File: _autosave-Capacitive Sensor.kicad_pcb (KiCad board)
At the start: 2 copper layers, 25 x 60.2 mm, 7 parts, among them J1 Conn_01x03, U1 TLC555

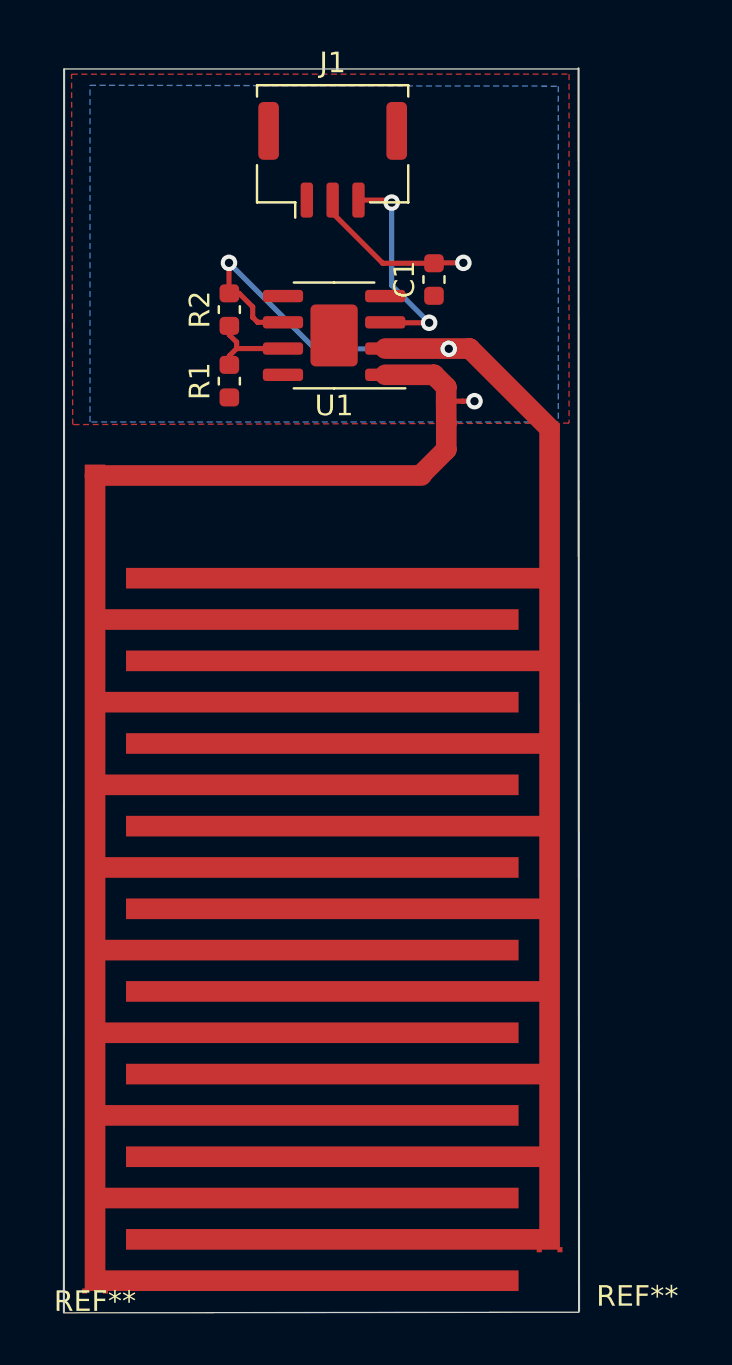
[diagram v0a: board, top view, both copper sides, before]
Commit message: update sensor
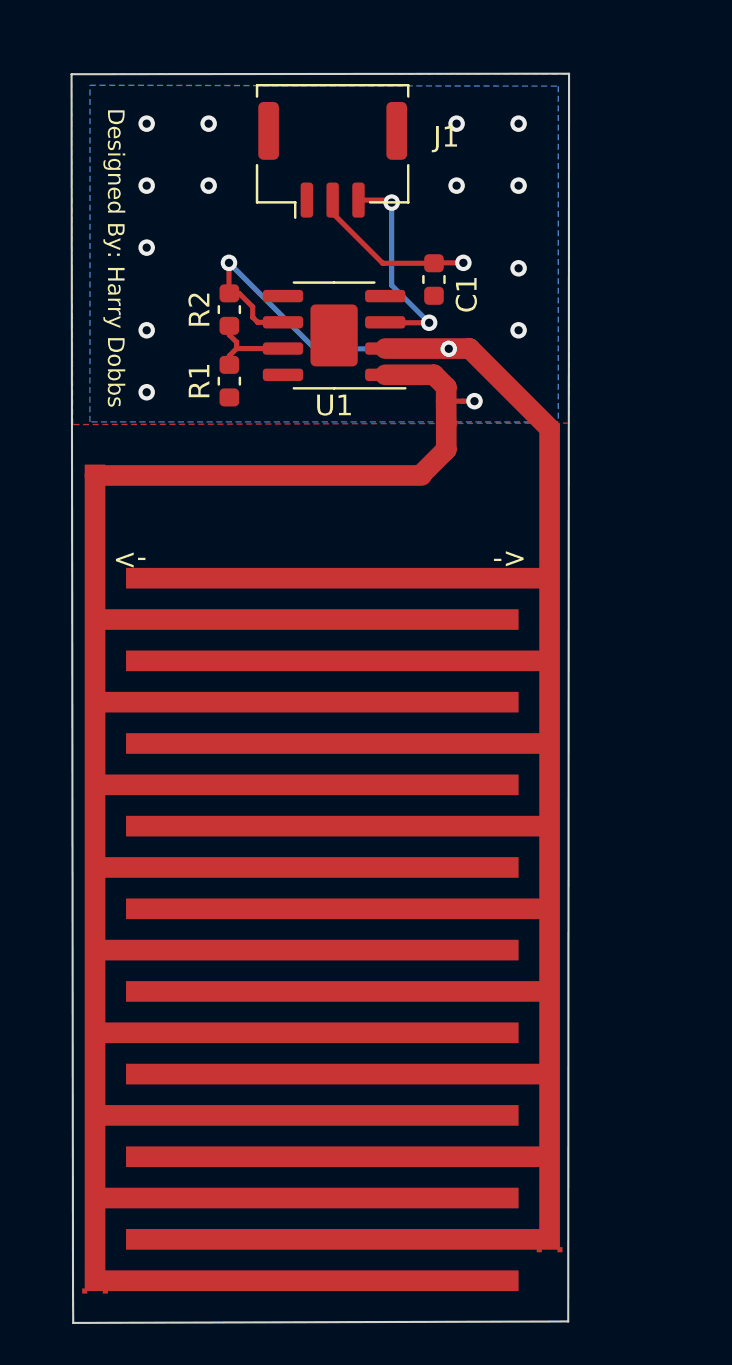
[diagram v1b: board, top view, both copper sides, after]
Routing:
- net C-: vias 2 -> 15
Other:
- board size 25 x 60.2 mm -> 24.1 x 60.5 mm
- board text added: "->"
- board text added: "Designed By: Harry Dobbs"
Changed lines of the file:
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@@
   (general
     (thickness 1.6)
-    (drawings 4)
-    (tracks 49)
+    (drawings 9)
+    (tracks 62)
     (zones 0)
     (modules 7)
@@
   )
   (setup
-    (last_trace_width 0.25)
+    (last_trace_width 1)
     (user_trace_width 0.25)
     (user_trace_width 1)
@@
     (solder_mask_min_width 0.25)
     (aux_axis_origin 0 0)
-    (visible_elements FFFBEF7F)
+    (visible_elements FFFFEF7F)
     (pcbplotparams
       (layerselection 0x010fc_ffffffff)
@@
   (module muwave_polygon (layer F.Cu)
     (at 160.5 141.5 180)
-    (fp_text reference REF** (at -4.25 -2.25) (layer F.SilkS)
-      (effects (font (size 1 1) (thickness 0.15)))
-    )
-    (fp_text value muwave_polygon (at -2.75 -3.5) (layer F.Fab)
+    (fp_text reference REF** (at 3.5 -2) (layer F.SilkS) hide
+      (effects (font (size 1 1) (thickness 0.15)))
+    )
+    (fp_text value muwave_polygon (at -10.78744 -4.41792) (layer F.Fab)
       (effects (font (size 1 1) (thickness 0.15)))
     )
@@
   (module muwave_polygon (layer F.Cu)
     (at 138.5 143.5)
-    (fp_text reference REF** (at 0 0.5) (layer F.SilkS)
-      (effects (font (size 1 1) (thickness 0.15)))
-    )
-    (fp_text value muwave_polygon (at 0 -0.5) (layer F.Fab)
+    (fp_text reference REF** (at 0 0.5) (layer F.SilkS) hide
+      (effects (font (size 1 1) (thickness 0.15)))
+    )
+    (fp_text value muwave_polygon (at -13 -1.5) (layer F.Fab)
       (effects (font (size 1 1) (thickness 0.15)))
     )
@@
     (tags "connector Molex CLIK-Mate side entry")
     (attr smd)
-    (fp_text reference J1 (at 0 -4.7) (layer F.SilkS)
+    (fp_text reference J1 (at 5.50896 -1.09968) (layer F.SilkS)
       (effects (font (size 1 1) (thickness 0.15)))
     )
@@
     (tags capacitor)
     (attr smd)
-    (fp_text reference C1 (at 0 -1.43 90) (layer F.SilkS)
+    (fp_text reference C1 (at -0.71638 1.6002 90) (layer F.SilkS)
       (effects (font (size 1 1) (thickness 0.15)))
     )
@@
       (effects (font (size 1 1) (thickness 0.15)))
     )
+    (fp_line (start -0.8 0.4) (end -0.8 -0.4) (layer F.Fab) (width 0.1))
+    (fp_line (start -0.8 -0.4) (end 0.8 -0.4) (layer F.Fab) (width 0.1))
+    (fp_line (start 0.8 -0.4) (end 0.8 0.4) (layer F.Fab) (width 0.1))
+    (fp_line (start 0.8 0.4) (end -0.8 0.4) (layer F.Fab) (width 0.1))
+    (fp_line (start -0.162779 -0.51) (end 0.162779 -0.51) (layer F.SilkS) (width 0.12))
+    (fp_line (start -0.162779 0.51) (end 0.162779 0.51) (layer F.SilkS) (width 0.12))
+    (fp_line (start -1.48 0.73) (end -1.48 -0.73) (layer F.CrtYd) (width 0.05))
+    (fp_line (start -1.48 -0.73) (end 1.48 -0.73) (layer F.CrtYd) (width 0.05))
+    (fp_line (start 1.48 -0.73) (end 1.48 0.73) (layer F.CrtYd) (width 0.05))
+    (fp_line (start 1.48 0.73) (end -1.48 0.73) (layer F.CrtYd) (width 0.05))
     (fp_text user %R (at 0.5 -1 90) (layer F.Fab)
       (effects (font (size 0.4 0.4) (thickness 0.06)))
     )
-    (fp_line (start 1.48 0.73) (end -1.48 0.73) (layer F.CrtYd) (width 0.05))
-    (fp_line (start 1.48 -0.73) (end 1.48 0.73) (layer F.CrtYd) (width 0.05))
-    (fp_line (start -1.48 -0.73) (end 1.48 -0.73) (layer F.CrtYd) (width 0.05))
-    (fp_line (start -1.48 0.73) (end -1.48 -0.73) (layer F.CrtYd) (width 0.05))
-    (fp_line (start -0.162779 0.51) (end 0.162779 0.51) (layer F.SilkS) (width 0.12))
-    (fp_line (start -0.162779 -0.51) (end 0.162779 -0.51) (layer F.SilkS) (width 0.12))
-    (fp_line (start 0.8 0.4) (end -0.8 0.4) (layer F.Fab) (width 0.1))
-    (fp_line (start 0.8 -0.4) (end 0.8 0.4) (layer F.Fab) (width 0.1))
-    (fp_line (start -0.8 -0.4) (end 0.8 -0.4) (layer F.Fab) (width 0.1))
-    (fp_line (start -0.8 0.4) (end -0.8 -0.4) (layer F.Fab) (width 0.1))
+    (pad 1 smd roundrect (at -0.7875 0 90) (size 0.875 0.95) (layers F.Cu F.Paste F.Mask) (roundrect_rratio 0.25)
+      (net 2 +3V3))
     (pad 2 smd roundrect (at 0.7875 0 90) (size 0.875 0.95) (layers F.Cu F.Paste F.Mask) (roundrect_rratio 0.25)
       (net 1 C-))
-    (pad 1 smd roundrect (at -0.7875 0 90) (size 0.875 0.95) (layers F.Cu F.Paste F.Mask) (roundrect_rratio 0.25)
-      (net 2 +3V3))
     (model ${KISYS3DMOD}/Capacitor_SMD.3dshapes/C_0603_1608Metric.wrl
       (at (xyz 0 0 0))
@@
     )
   )
-  (gr_line (start 136.99236 84.3534) (end 161.8996 84.3534) (layer Edge.Cuts) (width 0.05))
-  (gr_line (start 136.96696 144.55648) (end 161.91992 144.526) (layer Edge.Cuts) (width 0.05))
-  (gr_line (start 161.8996 84.32292) (end 161.925 144.47012) (layer Edge.Cuts) (width 0.1))
-  (gr_line (start 136.99236 144.50568) (end 137.00252 84.36864) (layer Edge.Cuts) (width 0.1))
+  (gr_text -> (at 140.18768 108.1532 180) (layer F.SilkS)
+    (effects (font (size 1 1) (thickness 0.15)))
+  )
+  (gr_text -> (at 158.56204 108.0262) (layer F.SilkS)
+    (effects (font (size 1 1) (thickness 0.15)))
+  )
+  (gr_text "Designed By: Harry Dobbs " (at 139.5 93.5 270) (layer F.SilkS)
+    (effects (font (size 0.8 0.8) (thickness 0.15)))
+  )
+  (gr_line (start 137.44448 145.04416) (end 137.43432 143.62176) (layer Edge.Cuts) (width 0.1))
+  (gr_line (start 161.40176 144.97304) (end 137.44448 145.04416) (layer Edge.Cuts) (width 0.1))
+  (gr_line (start 161.4424 84.582) (end 161.40176 144.97304) (layer Edge.Cuts) (width 0.1))
+  (gr_line (start 137.3632 84.6074) (end 161.4424 84.582) (layer Edge.Cuts) (width 0.1))
+  (gr_line (start 137.43432 143.59128) (end 137.3632 84.6074) (layer Edge.Cuts) (width 0.1))
+  (gr_line (start 137.43432 143.62176) (end 137.43432 143.59128) (layer Edge.Cuts) (width 0.1))
   (segment (start 152.5375 99.1625) (end 152.545 99.155) (width 0.25) (layer F.Cu) (net 1))
   (segment (start 152.545 99.155) (end 154.905 99.155) (width 1) (layer F.Cu) (net 1))
@@
   (segment (start 155.49372 100.4316) (end 155.5 101.5) (width 1) (layer F.Cu) (net 1))
   (segment (start 155.5 99.75) (end 155.49372 100.4316) (width 1) (layer F.Cu) (net 1))
+  (via (at 141 87) (size 0.8) (drill 0.4) (layers F.Cu B.Cu) (net 1))
+  (via (at 141 90) (size 0.8) (drill 0.4) (layers F.Cu B.Cu) (net 1))
+  (via (at 141 93) (size 0.8) (drill 0.4) (layers F.Cu B.Cu) (net 1))
+  (via (at 141 97) (size 0.8) (drill 0.4) (layers F.Cu B.Cu) (net 1))
+  (via (at 144 87) (size 0.8) (drill 0.4) (layers F.Cu B.Cu) (net 1))
+  (via (at 144 90) (size 0.8) (drill 0.4) (layers F.Cu B.Cu) (net 1))
+  (via (at 156 87) (size 0.8) (drill 0.4) (layers F.Cu B.Cu) (net 1))
+  (via (at 159 87) (size 0.8) (drill 0.4) (layers F.Cu B.Cu) (net 1))
+  (via (at 159 90) (size 0.8) (drill 0.4) (layers F.Cu B.Cu) (net 1))
+  (via (at 156 90) (size 0.8) (drill 0.4) (layers F.Cu B.Cu) (net 1))
+  (via (at 159 94) (size 0.8) (drill 0.4) (layers F.Cu B.Cu) (net 1))
+  (via (at 159 97) (size 0.8) (drill 0.4) (layers F.Cu B.Cu) (net 1))
+  (via (at 141 100) (size 0.8) (drill 0.4) (layers F.Cu B.Cu) (net 1))
   (via (at 152.8572 90.82024) (size 0.8) (drill 0.4) (layers F.Cu B.Cu) (net 3))
   (via (at 154.67076 96.63684) (size 0.8) (drill 0.4) (layers F.Cu B.Cu) (net 3))
